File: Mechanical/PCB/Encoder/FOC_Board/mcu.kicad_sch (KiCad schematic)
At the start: 54 parts, among them IC2 TPS563200DDCR, J1 CAN_IN, J2 CAN_OUT, J3 XT30PW-M, J7 SWD, J8 UART, J9 HALL, U2 STM32G431CBUx, U4 ME6211C33M5, U5 TJA1051T-3, Y2 8MHz

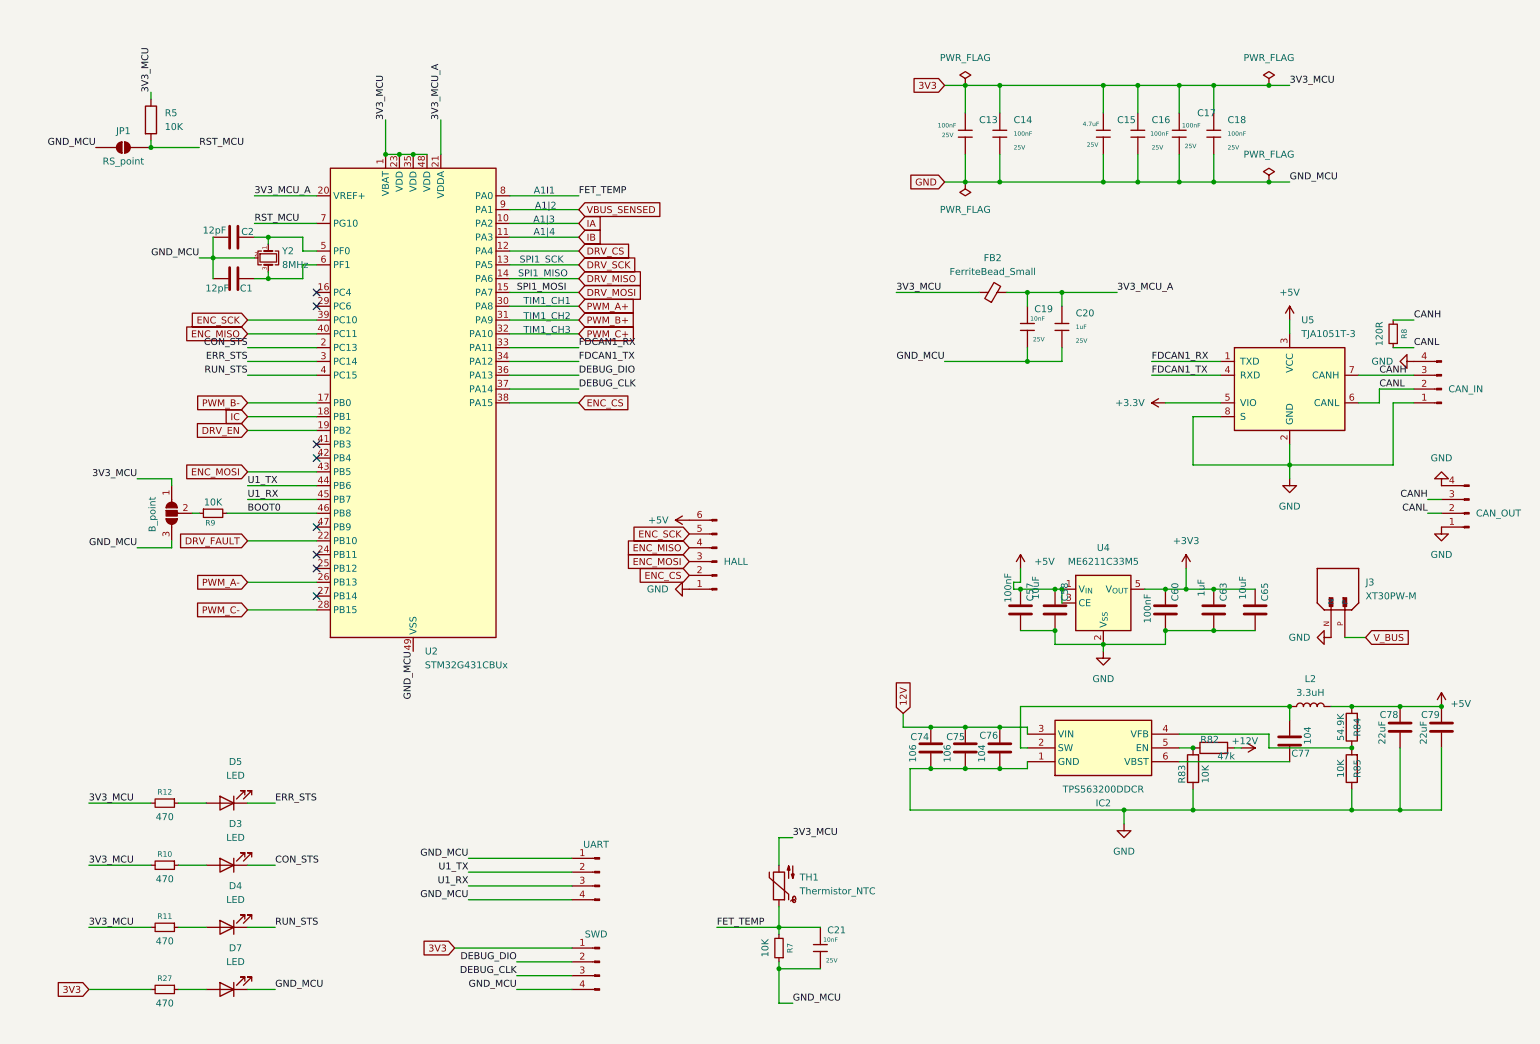
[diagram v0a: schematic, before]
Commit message: OPEN LOOP FOC
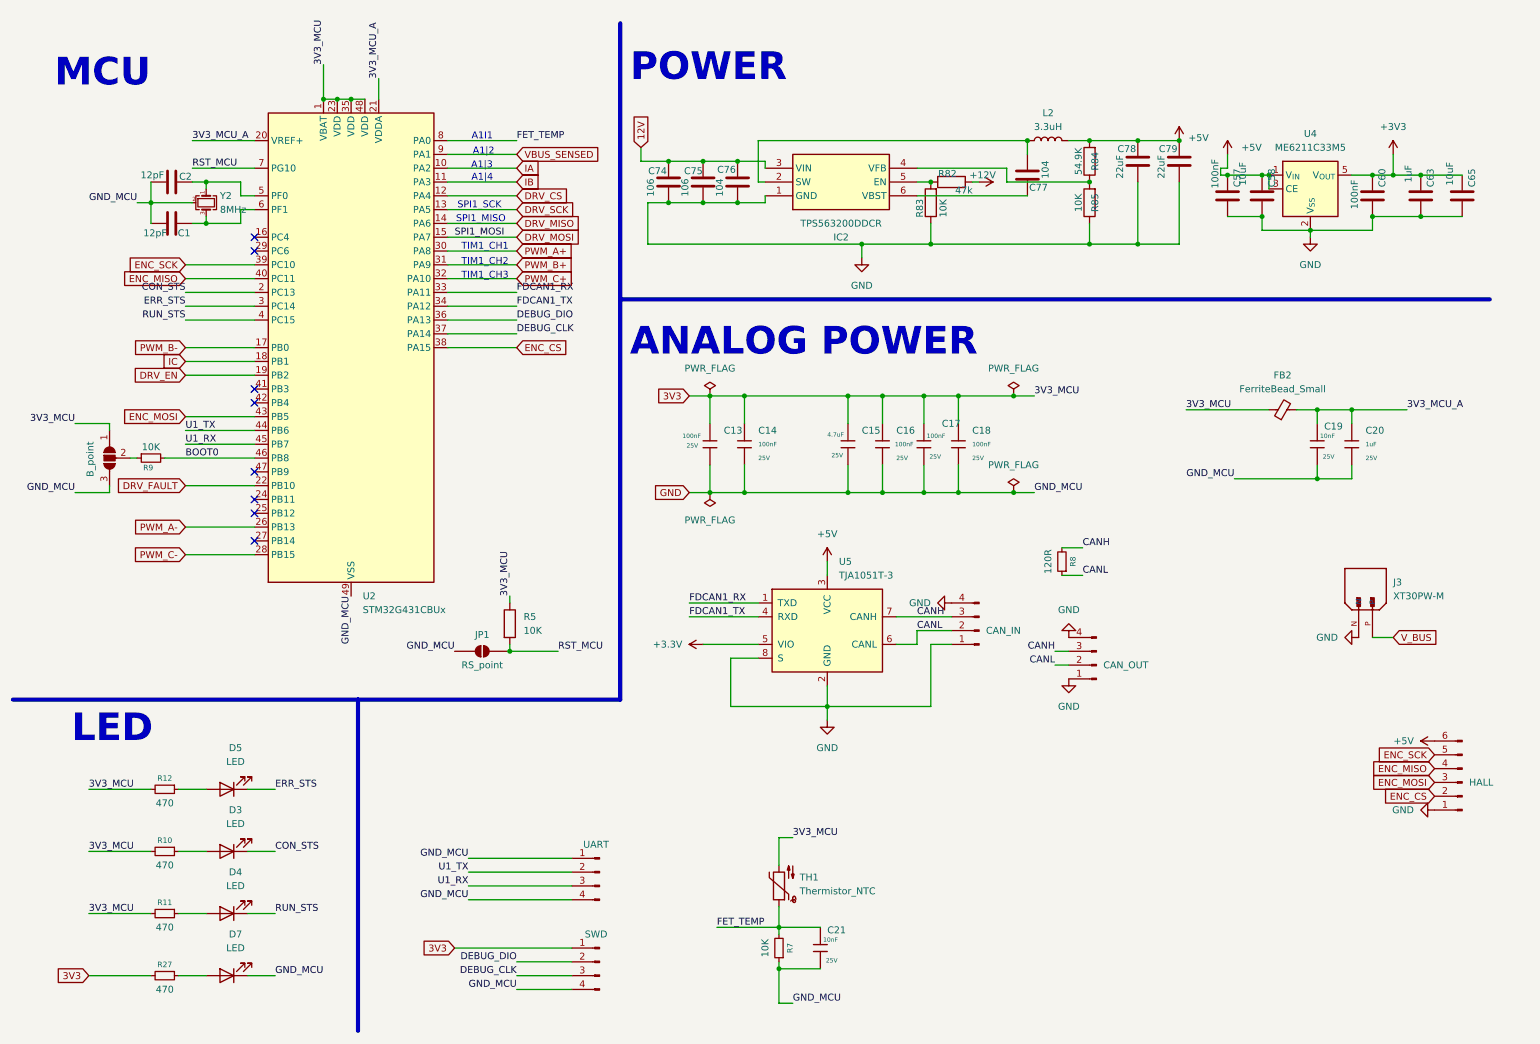
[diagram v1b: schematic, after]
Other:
- note added: "ANALOG POWER"
- note added: "LED"
- note added: "MCU"
- note added: "POWER"
- moved on the sheet: C1, C13, C14, C15, C16, C17, C18, C19, C2, C20, C57, C58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
